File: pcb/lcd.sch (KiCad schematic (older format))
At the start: 37 parts, among them J500 FPC_18P_1.0MM, Q500 IRLML6402, U100 MCIMX7S5EVM08SC, U500 XC2C32A, U501 ADP5075, U502 LM324

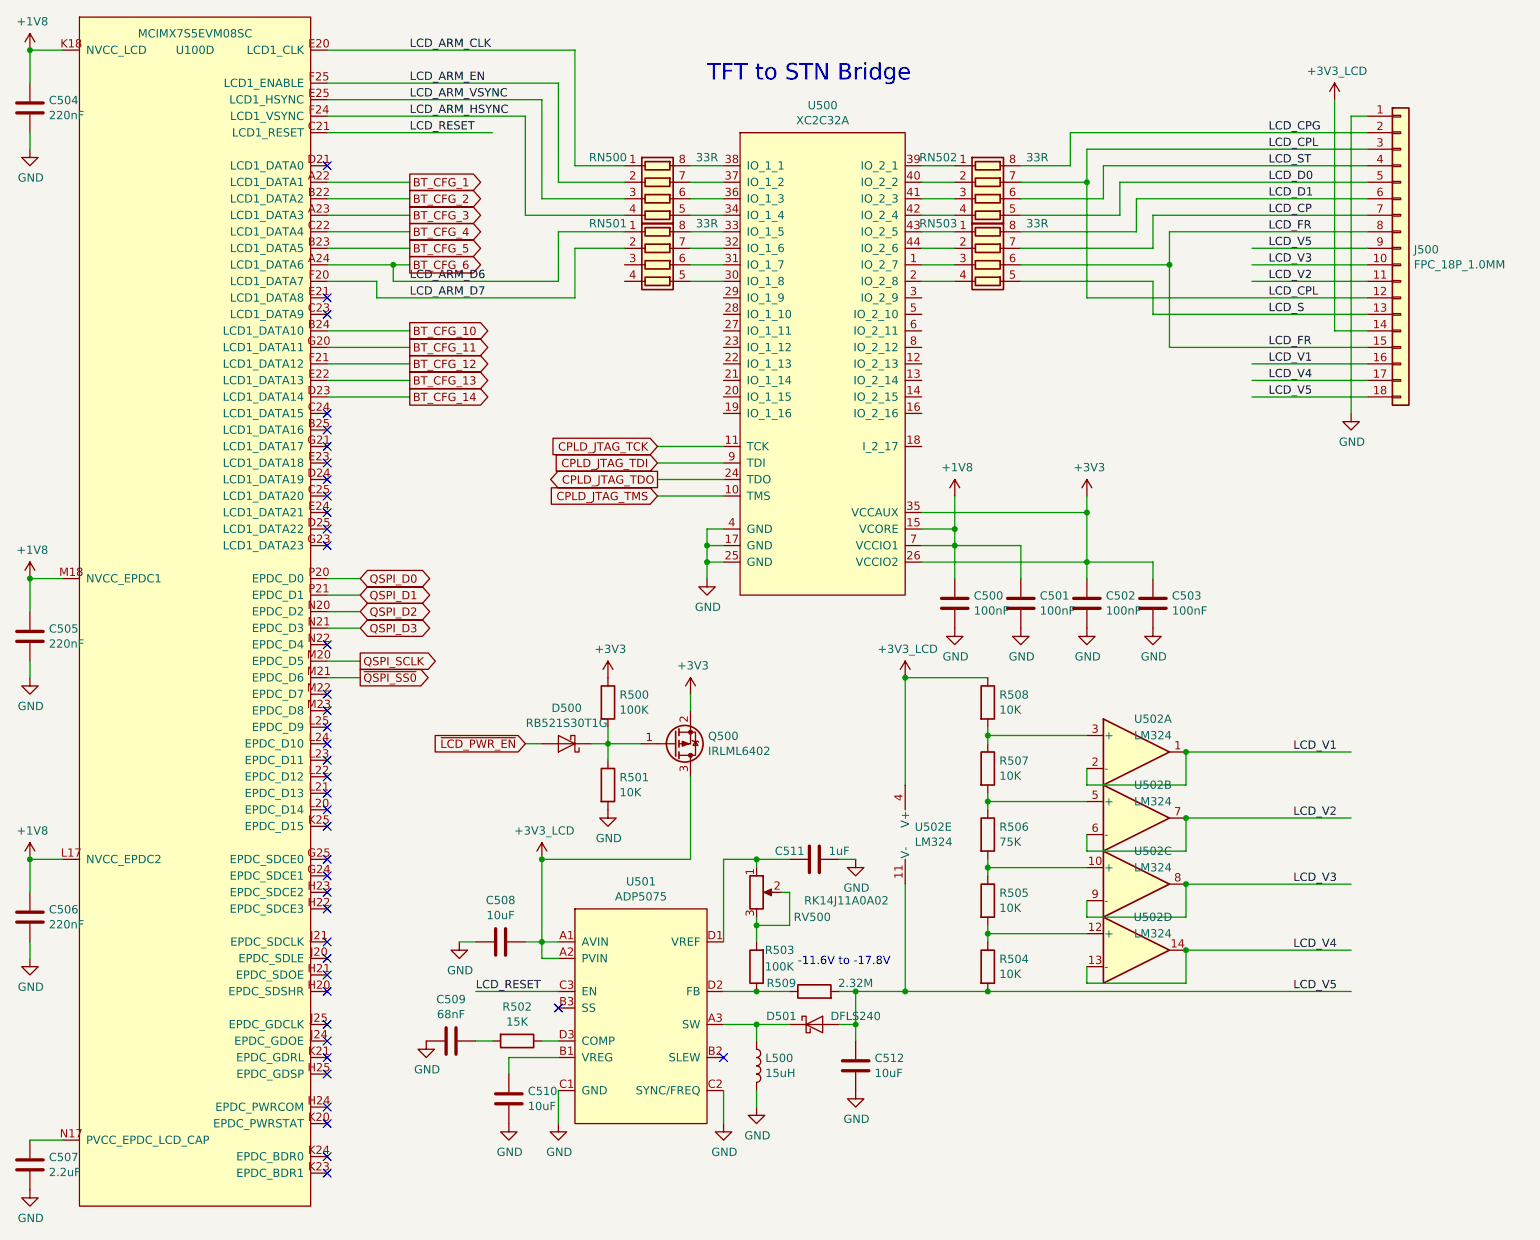
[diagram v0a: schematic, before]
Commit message: pcb: working on layout
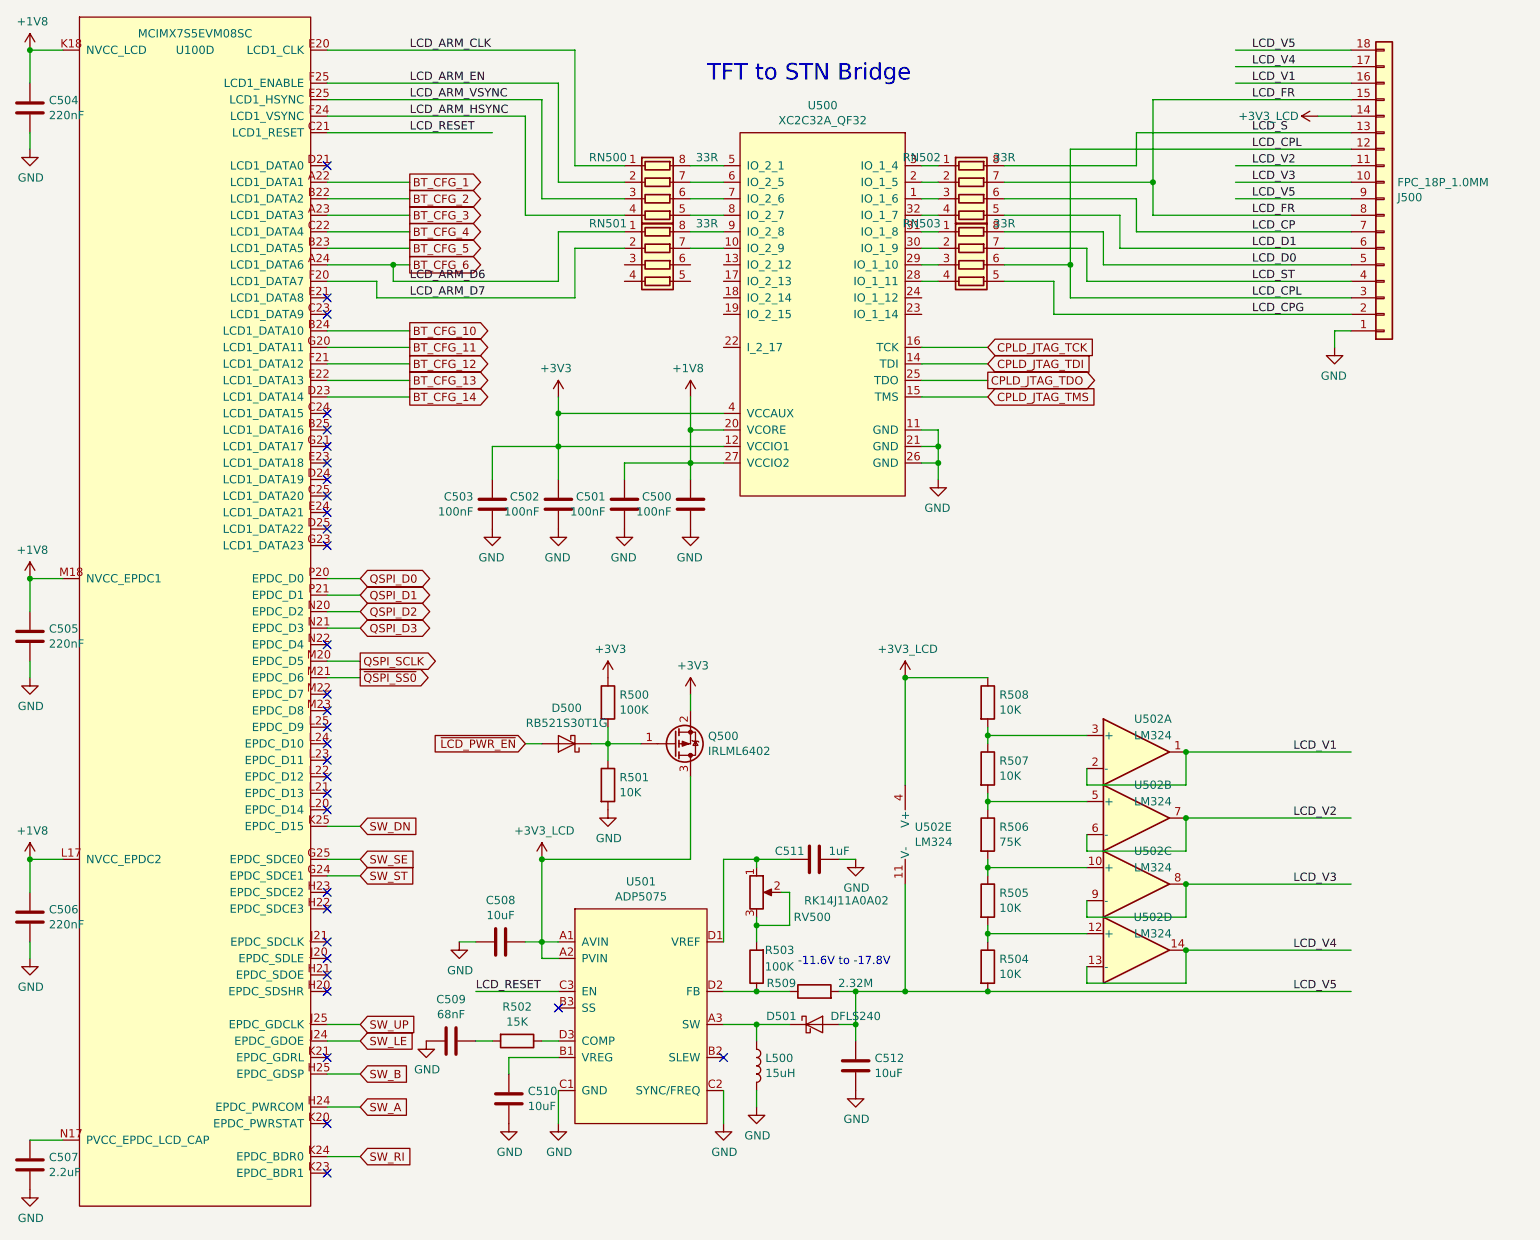
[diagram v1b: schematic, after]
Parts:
- removed U500: XC2C32A, Package_QFP:LQFP-44_10x10mm_P0.8mm, symbol symbols:XC2C32A
- added U500: XC2C32A_QF32, Package_DFN_QFN:QFN-32-1EP_5x5mm_P0.5mm_EP3.1x3.1mm, symbol symbols:XC2C32A_QF32
- L500: footprint Inductor_SMD:L_Vishay_IHLP-4040 -> Inductor_SMD:L_Vishay_IHLP-1212
- U502: footprint Package_SO:SOIC-16_3.9x9.9mm_P1.27mm -> Package_SO:TSSOP-14_4.4x5mm_P0.65mm
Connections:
- net labels added: SW_A, SW_B, SW_DN, SW_LE, SW_RI, SW_SE, SW_ST, SW_UP
- wire segments 203 -> 208
- no-connect marks 40 -> 32
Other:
- moved on the sheet: C500, C501, C502, C503, J500, RN502, RN503
